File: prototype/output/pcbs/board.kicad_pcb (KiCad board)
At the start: 2 copper layers, 143.9 x 111.2 mm, 52 parts

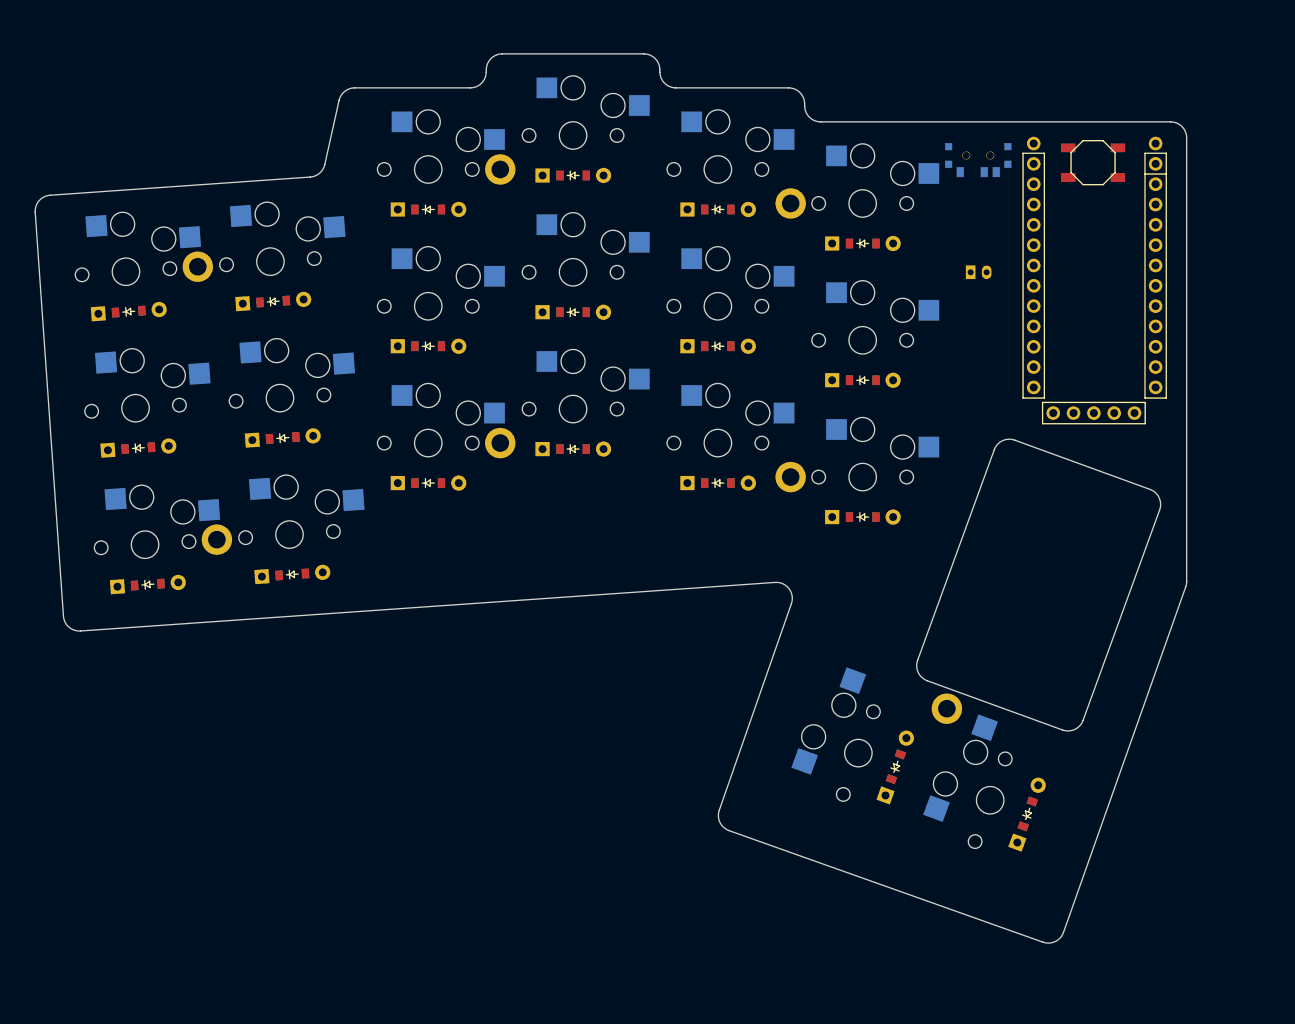
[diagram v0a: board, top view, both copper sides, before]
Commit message: cleanup
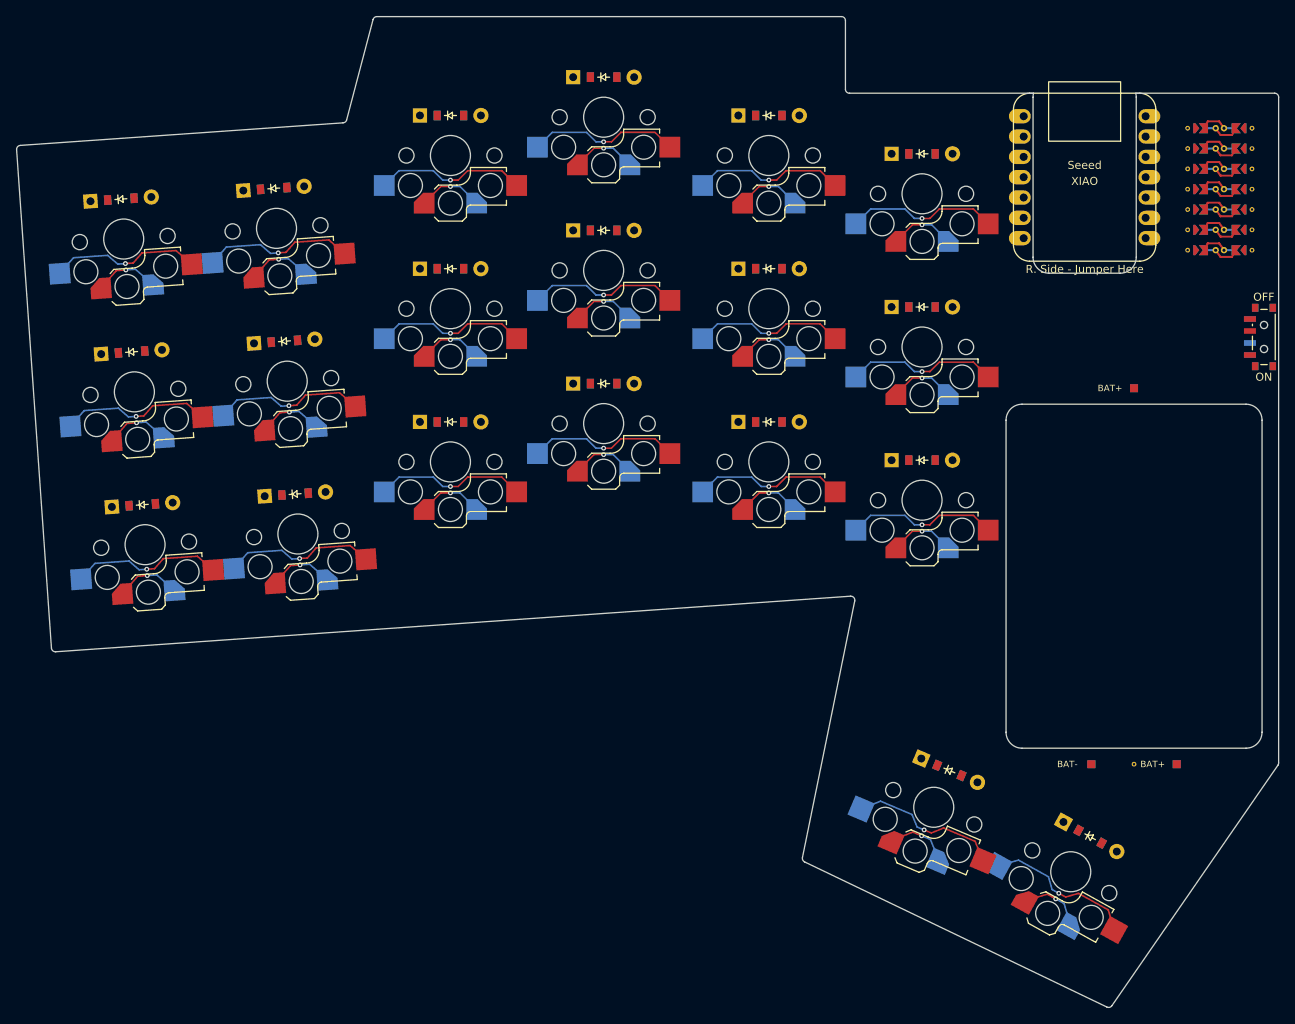
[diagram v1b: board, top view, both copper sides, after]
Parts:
- removed the ? at (118.7, -34.9)
- removed B1: , E73:SW_TACT_ALPS_SKQGABE010
- removed DISP1: , ceoloide:display_nice_view
- removed H1, H2, H3, H4, H5, H6, H7: , ceoloide:mounting_hole_plated
- removed JST1: , JST_PH_S2B-PH-K_02x2.00mm_Angled
- removed T1: , E73:SPDT_C128955
- added ?: , xiao-ble-tht, F.Cu at (117.4, -45.9)
- added PAD1: , SMDPad, F.Cu at (123.6, -19.6)
- added PAD2: , SMDPad, F.Cu at (129.0, 27.4)
- added PAD3: , SMDPad, F.Cu at (118.3, 27.4)
- added PWR1: , ceoloide:power_switch_smd_side, F.Cu at (139.8, -26.0)
- added REF**: VIA-0.6mm, VIA-0.6mm, F.Cu at (123.6, 27.4)
- S1, S10, S11, S12, S13, S14, S15, S16, S17, S18, S19, S2, S20, S3, S4, S5, S6, S7, S8, S9: footprint PG1350 -> ceoloide:switch_choc_v1_v2; moved to B.Cu
- moved D6 14.1 mm to (16.1, -44.5)
- moved D3 14.1 mm to (-3.02, -43.2)
- moved S20 13.5 mm to (115.7, 40.9), turned to 151 degrees
- moved D18 13.4 mm to (97.1, -48.9)
- moved D15 13.4 mm to (78.0, -53.6)
- moved D12 12.9 mm to (57.3, -58.4)
- moved D5 12.1 mm to (17.4, -25.4)
- moved D9 12.1 mm to (38.2, -53.6)
- moved D2 12.1 mm to (-1.68, -24.1)
- moved D17 11.8 mm to (97.1, -29.7)
- moved D14 11.6 mm to (78.0, -34.5)
- moved S19 11.6 mm to (98.6, 32.8), turned to 157 degrees
- moved D11 10.9 mm to (57.3, -39.3)
- moved D16 10.3 mm to (97.1, -10.6)
- moved D8 10.1 mm to (38.2, -34.5)
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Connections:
- net P009 renamed P7
- net P010 renamed P8
- net P011 renamed P4
- net P022 renamed P1
- net P024 renamed P2
- net P100 renamed P3
- net P104 renamed P5
- net P106 renamed P6
- net P111 renamed P9
- net P113 renamed P10
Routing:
- net (no net): track 0.00 -> 68.6 mm
- net P6: track 0.00 -> 33.1 mm, vias 0 -> 4
- net P5: track 0.00 -> 33.1 mm, vias 0 -> 4
- net P2: track 0.00 -> 24.8 mm, vias 0 -> 3
- net P1: track 0.00 -> 24.8 mm, vias 0 -> 3
- net P4: track 0.00 -> 24.8 mm, vias 0 -> 3
- net P3: track 0.00 -> 24.8 mm, vias 0 -> 3
- net outer_cluster: track 0.00 -> 19.1 mm, vias 0 -> 1
- net inner_top: track 0.00 -> 19.1 mm, vias 0 -> 1
- net index_top: track 0.00 -> 19.1 mm, vias 0 -> 1
- net inner_bottom: track 0.00 -> 19.1 mm, vias 0 -> 1
- net inner_home: track 0.00 -> 19.1 mm, vias 0 -> 1
- net index_home: track 0.00 -> 19.1 mm, vias 0 -> 1
- net index_bottom: track 0.00 -> 19.1 mm, vias 0 -> 1
- net middle_bottom: track 0.00 -> 19.1 mm, vias 0 -> 1
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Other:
- board size 143.9 x 111.2 mm -> 157.8 x 123.9 mm
